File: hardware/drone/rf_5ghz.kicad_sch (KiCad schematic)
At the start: 25 parts, among them J5 Conn_01x06_Pin, U23 MM8030_2610RJ3, U7 CC3350, U8 DPX167125DT-8197B1, U9 DEA162450BT-1295A1, Y1 Crystal_GND24

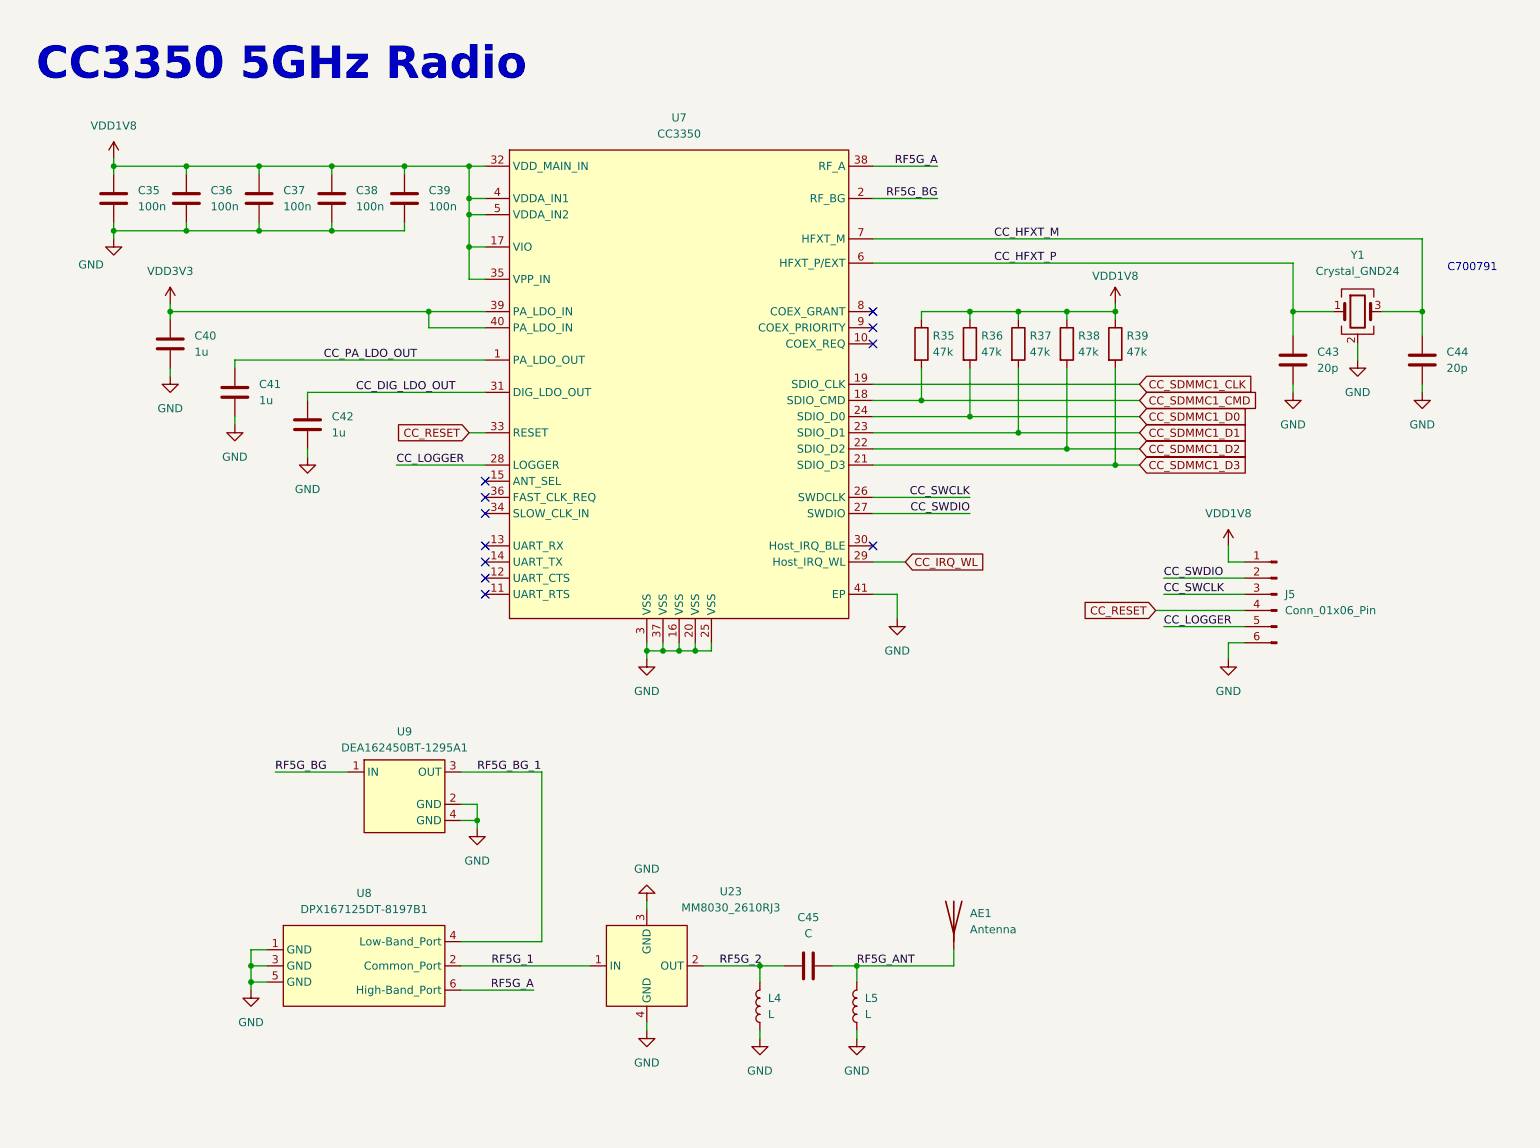
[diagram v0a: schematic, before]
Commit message: Small cleanup and more power routing
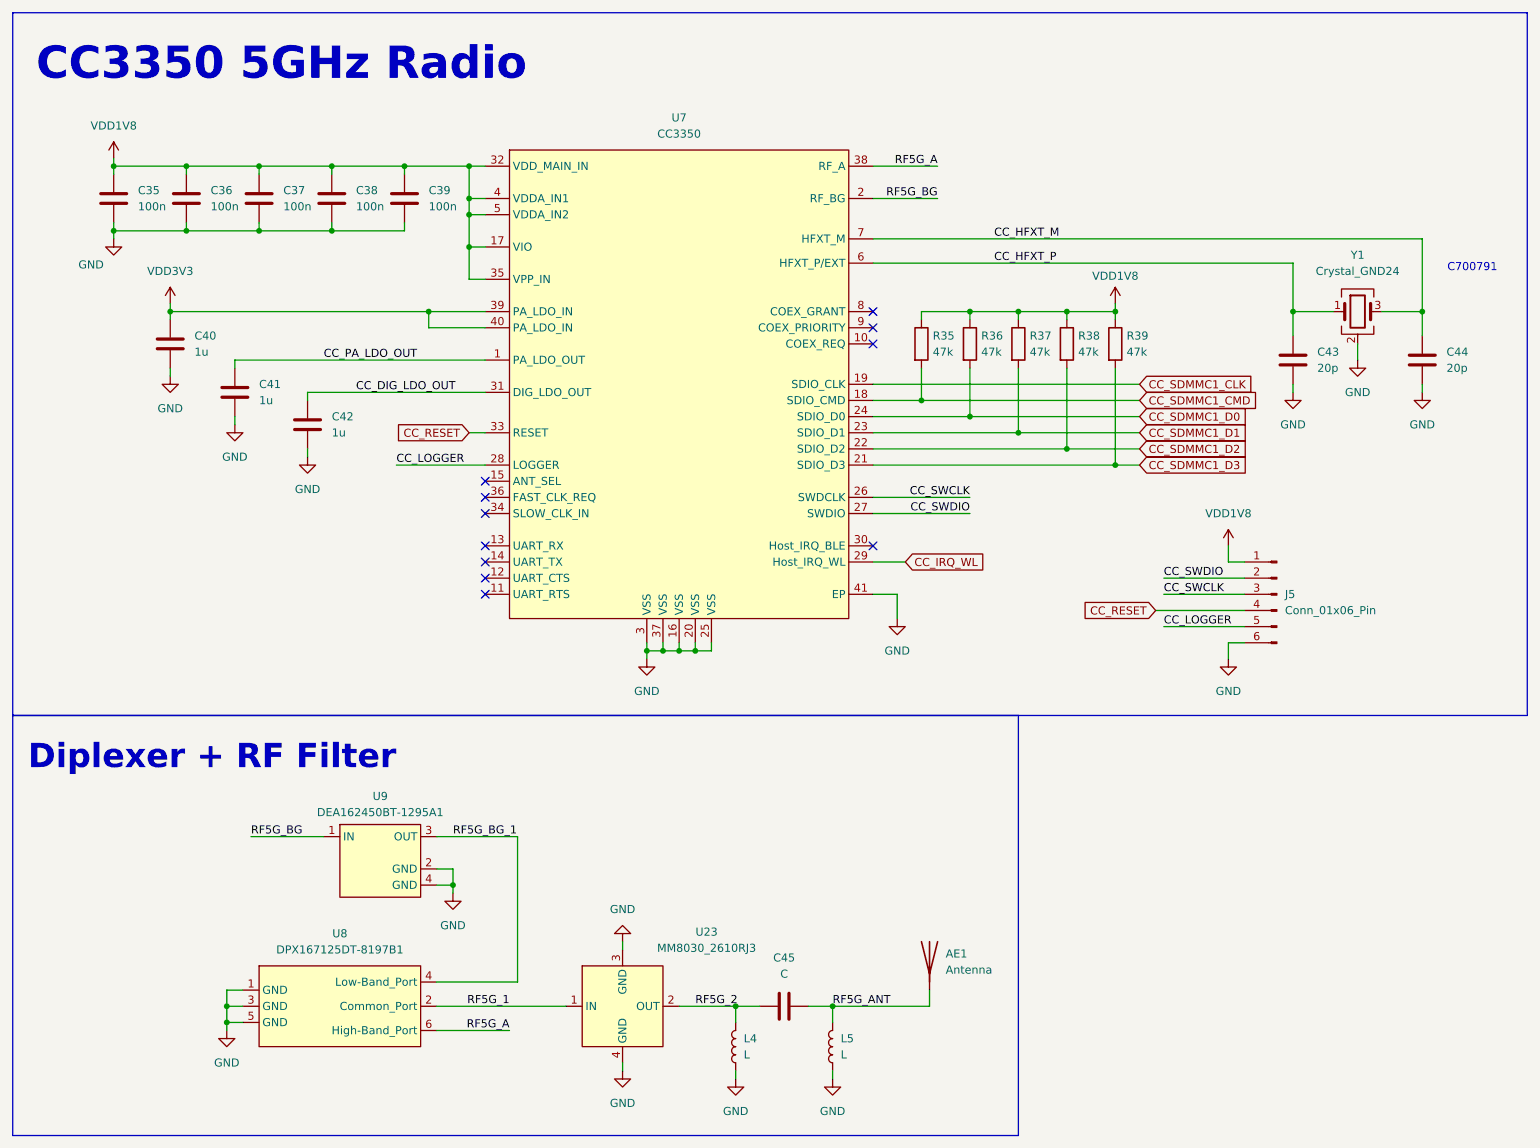
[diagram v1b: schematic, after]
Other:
- note added: "Diplexer + RF Filter"
- moved on the sheet: AE1, C45, L4, L5, U23, U8, U9
